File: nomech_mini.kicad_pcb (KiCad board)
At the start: 2 copper layers, 63 x 63 mm, 9 parts

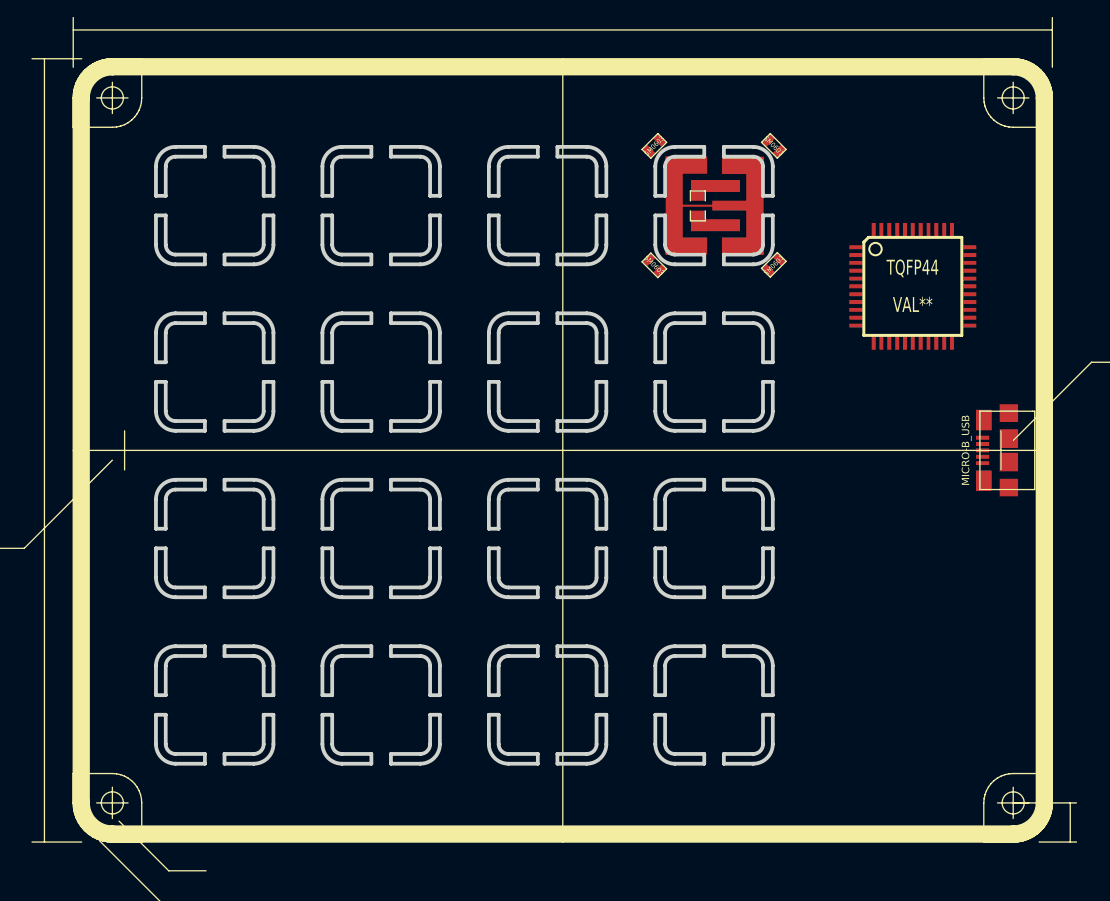
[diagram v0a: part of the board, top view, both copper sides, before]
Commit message: starting schematic, adjusting pcb
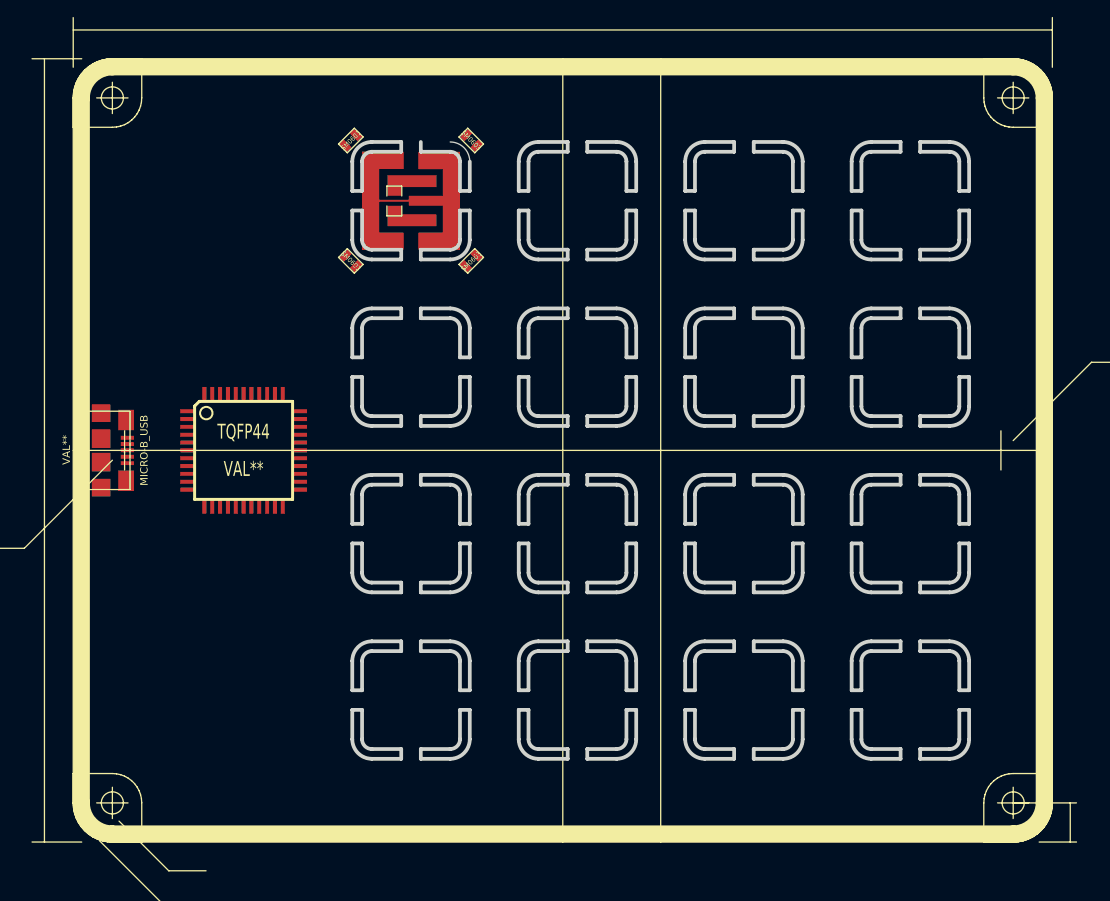
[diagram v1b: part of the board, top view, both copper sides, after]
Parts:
- added 80x80: 80mm, dp_pcb-DP8080_V1_drawing, F.Cu at (98.8, 154.8)
- DP10080_v1: renamed from 80mm; value 100mm -> 100x80mm
- moved MICRO-B_USB 95.6 mm to (80.2, 114.8), turned to 270 degrees
- moved TQFP44 70.4 mm to (96.2, 114.8)
- moved SM0603 31.0 mm to (107.1, 83.1)
- moved cap-electrode_10mm 31.0 mm to (113.2, 89.2)
- moved SM0603 31.0 mm to (107.1, 95.4)
- moved SM0603 30.9 mm to (119.4, 83.1)
- moved SM0603 30.9 mm to (119.4, 95.4)
